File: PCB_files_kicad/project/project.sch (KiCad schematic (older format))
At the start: 23 parts, among them J1 Conn_01x08_Female, J2 S1, J3 S2, J4 Conn_01x08_Female, J5 Display, J6 HC06, U1 M24C02

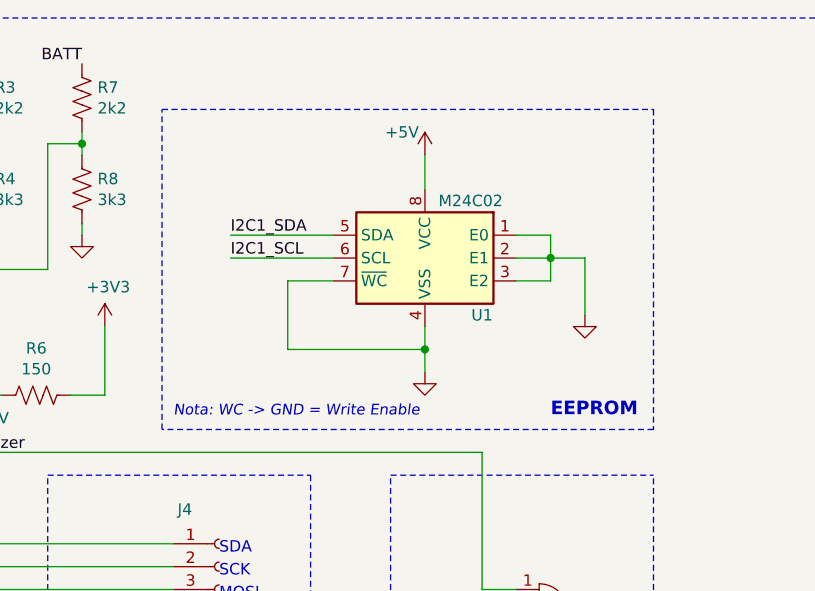
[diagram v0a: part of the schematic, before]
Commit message: Minor changes
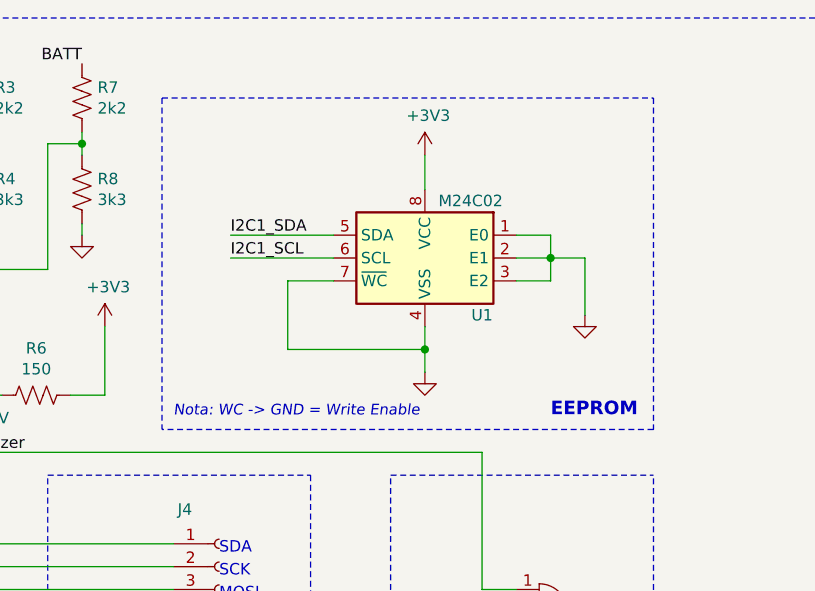
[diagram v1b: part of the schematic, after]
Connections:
- net +3V3: now also U1.8 (VCC)
- net +5V: no longer U1.8 (VCC)
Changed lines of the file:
@@
 	3200 1950 4000 1950
 $Comp
-L power:+5V #PWR02
+L power:+5V #PWR03
 U 1 1 613FF598
 P 3300 1750
-F 0 "#PWR02" H 3300 1600 50  0001 C CNN
+F 0 "#PWR03" H 3300 1600 50  0001 C CNN
 F 1 "+5V" H 3200 1850 50  0000 C CNN
 F 2 "" H 3300 1750 50  0001 C CNN
@@
 $EndComp
 $Comp
-L power:+5V #PWR03
+L power:+5V #PWR04
 U 1 1 613FFC5D
 P 3300 2350
-F 0 "#PWR03" H 3300 2200 50  0001 C CNN
+F 0 "#PWR04" H 3300 2200 50  0001 C CNN
 F 1 "+5V" H 3200 2450 50  0000 C CNN
 F 2 "" H 3300 2350 50  0001 C CNN
@@
 $EndComp
 $Comp
-L power:GND #PWR04
+L power:GND #PWR05
 U 1 1 6140B0AA
 P 3500 2150
-F 0 "#PWR04" H 3500 1900 50  0001 C CNN
+F 0 "#PWR05" H 3500 1900 50  0001 C CNN
 F 1 "GND" H 3505 1977 50  0001 C CNN
 F 2 "" H 3500 2150 50  0001 C CNN
@@
 	4000 1950 4000 2350
 $Comp
-L power:GND #PWR05
+L power:GND #PWR06
 U 1 1 61409F32
 P 3500 2750
-F 0 "#PWR05" H 3500 2500 50  0001 C CNN
+F 0 "#PWR06" H 3500 2500 50  0001 C CNN
 F 1 "GND" H 3505 2577 50  0001 C CNN
 F 2 "" H 3500 2750 50  0001 C CNN
@@
 Wire Notes Line
 	9300 2900 7150 2900
-Wire Notes Line
-	7150 2900 7150 1500
-Wire Notes Line
-	7150 1500 9300 1500
-Wire Notes Line
-	9300 1500 9300 2900
 Wire Wire Line
 	8300 1850 8300 1700
 Wire Wire Line
 	8300 2450 8300 2550
-$Comp
-L power:+5V #PWR023
-U 1 1 6161D033
-P 8300 1700
-F 0 "#PWR023" H 8300 1550 50  0001 C CNN
-F 1 "+5V" H 8200 1800 50  0000 C CNN
-F 2 "" H 8300 1700 50  0001 C CNN
-F 3 "" H 8300 1700 50  0001 C CNN
-	1    8300 1700
-	1    0    0    -1
-$EndComp
 $Comp
 L power:GND #PWR024
@@
 $EndComp
 $Comp
-L power:PWR_FLAG #FLG02
+L power:PWR_FLAG #FLG01
 U 1 1 61497233
 P 3950 7450
-F 0 "#FLG02" H 3950 7525 50  0001 C CNN
+F 0 "#FLG01" H 3950 7525 50  0001 C CNN
 F 1 "PWR_FLAG" H 3950 7623 50  0000 C CNN
 F 2 "" H 3950 7450 50  0001 C CNN
@@
 	3250 7500 3250 7050
 $Comp
-L power:+3V3 #PWR0101
+L power:+3V3 #PWR02
 U 1 1 61603C70
 P 3250 7050
-F 0 "#PWR0101" H 3250 6900 50  0001 C CNN
+F 0 "#PWR02" H 3250 6900 50  0001 C CNN
 F 1 "+3V3" H 3265 7223 50  0000 C CNN
 F 2 "" H 3250 7050 50  0001 C CNN
@@
 	1    0    0    -1
 $EndComp
+$Comp
+L power:+3V3 #PWR?
+U 1 1 6158619C
+P 8300 1700
+F 0 "#PWR?" H 8300 1550 50  0001 C CNN
+F 1 "+3V3" H 8315 1873 50  0000 C CNN
+F 2 "" H 8300 1700 50  0001 C CNN
+F 3 "" H 8300 1700 50  0001 C CNN
+	1    8300 1700
+	1    0    0    -1
+$EndComp
+Wire Notes Line
+	7150 1450 9300 1450
+Wire Notes Line
+	9300 1450 9300 2900
+Wire Notes Line
+	7150 1450 7150 2900
 $EndSCHEMATC
